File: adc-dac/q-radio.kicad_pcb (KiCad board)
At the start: 6 copper layers, 120 x 75 mm, 53 parts, among them U18 MAX5865, U3 GT4227, U34 GT4227, U35 GT4227, U36 74LVC1G86, U8 GT4227

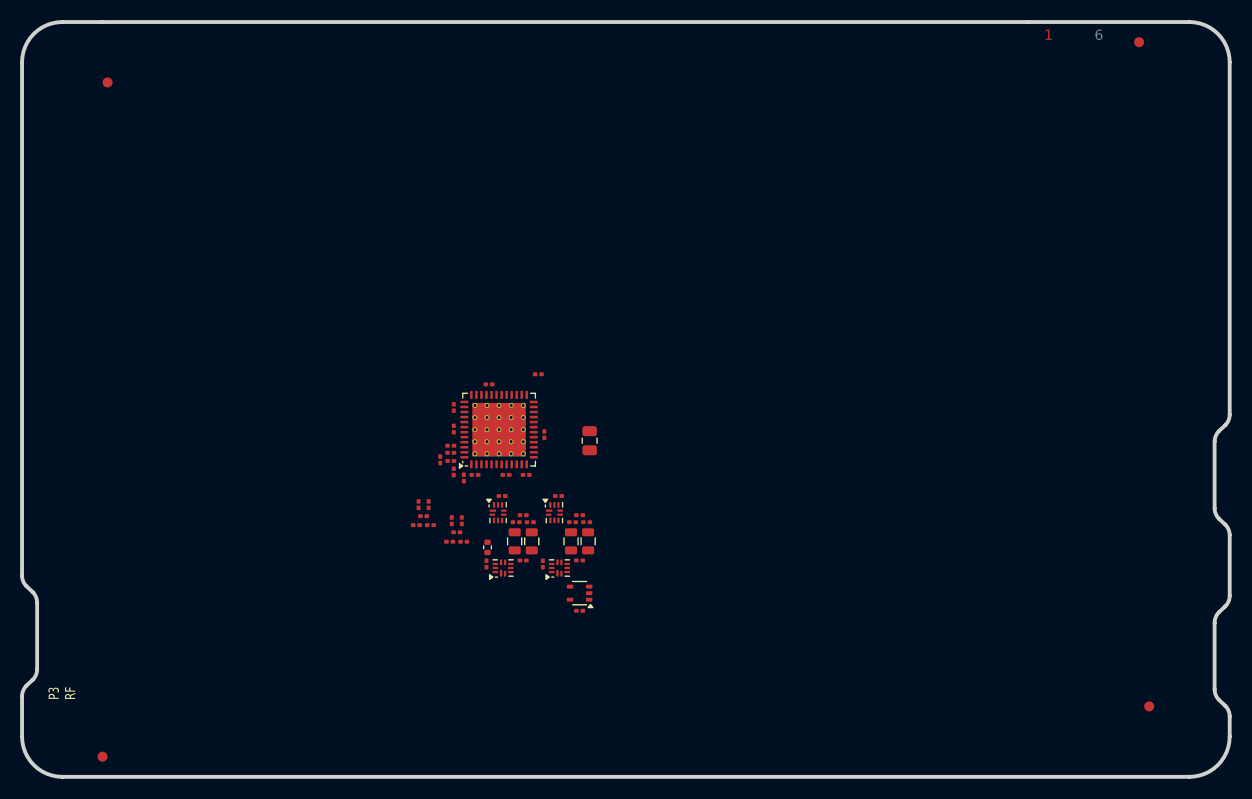
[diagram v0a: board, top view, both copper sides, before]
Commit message: All sub-modules added to child projects
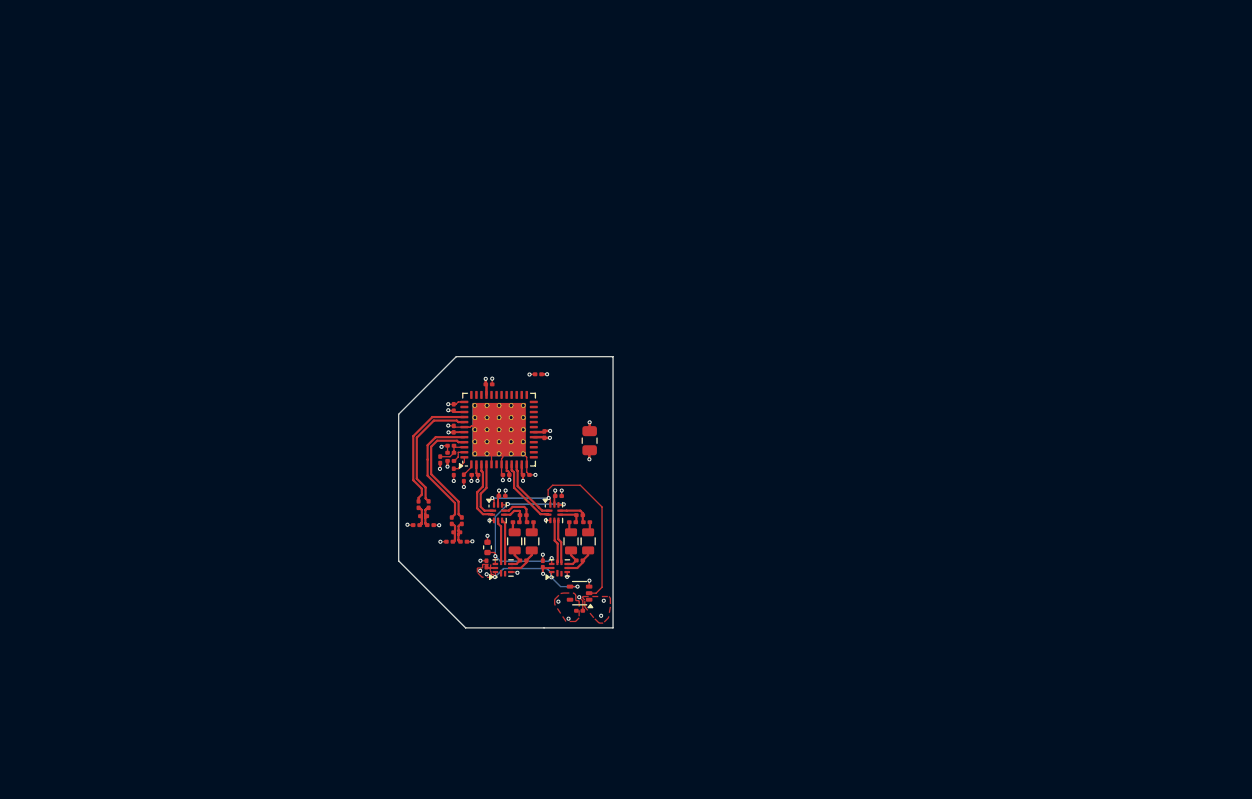
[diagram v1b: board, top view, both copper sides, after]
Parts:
- removed FID1, FID2, FID3, FID4: Fiducial_1mm_Mask2mm, Fiducial:Fiducial_1mm_Mask2mm
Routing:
- net GND: track 0.00 -> 35.3 mm, vias 0 -> 28
- net /ADC, DAC/AA_EN: track 0.00 -> 24.0 mm, vias 0 -> 2
- net /ADC, DAC/~{BB_EN}: track 0.00 -> 21.3 mm, vias 0 -> 4
- net VAA: track 0.00 -> 16.1 mm, vias 0 -> 16
- net /ADC, DAC/QD+: track 0.00 -> 12.8 mm
- net /ADC, DAC/ID-: track 0.00 -> 12.4 mm
- net /ADC, DAC/QD-: track 0.00 -> 12.3 mm
- net /ADC, DAC/ID+: track 0.00 -> 11.9 mm
- net /ADC, DAC/~{AA_EN}: track 0.00 -> 11.3 mm, vias 0 -> 3
- net /ADC, DAC/QA-: track 0.00 -> 6.97 mm
- net /ADC, DAC/IA+: track 0.00 -> 6.43 mm
- net /ADC, DAC/QA+: track 0.00 -> 6.35 mm
- net /ADC, DAC/IA-: track 0.00 -> 5.82 mm
- net /ADC, DAC/AA_BYPASS_Q+: track 0.00 -> 4.31 mm
- net /ADC, DAC/AA_BYPASS_Q-: track 0.00 -> 4.31 mm
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- added copper zone on In2.Cu, net 3V3FPGA
- added copper zone on In1.Cu, net GND
- added copper zone on In4.Cu, net GND
- added copper zone on F.Cu, net VAA
- added copper zone on In2.Cu, net VAA
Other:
- board size 120 x 75 mm -> 21.3 x 26.9 mm
- board text removed: "1"
- board text removed: "2"
- board text removed: "3"
- board text removed: "4"
- board text removed: "5"
- board text removed: "6"
- board text removed: "P3 RF"
